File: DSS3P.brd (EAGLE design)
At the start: 399.7 x 251.8 mm, 299 parts, among them J1 J7MM

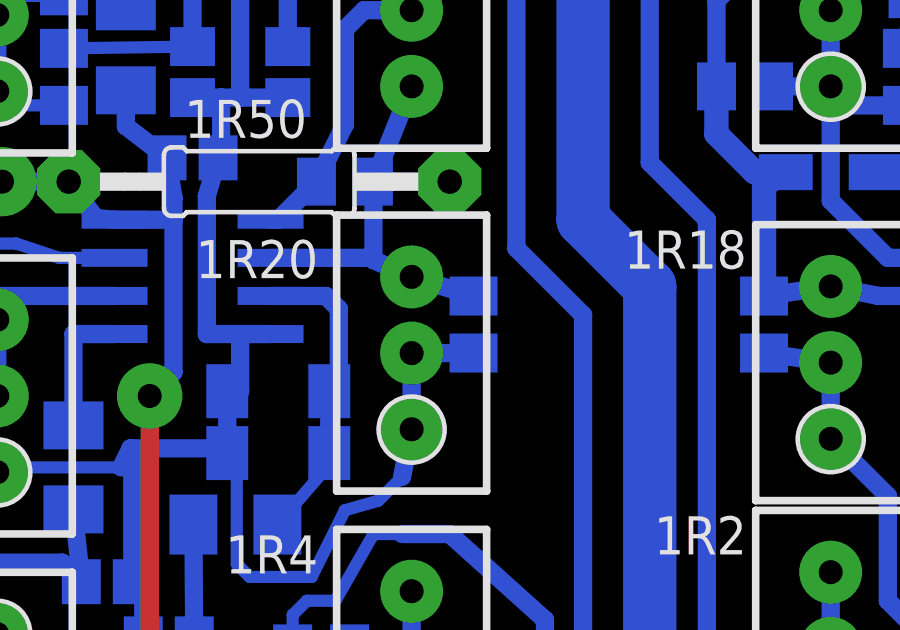
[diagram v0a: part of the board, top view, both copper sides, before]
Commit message: lab bot
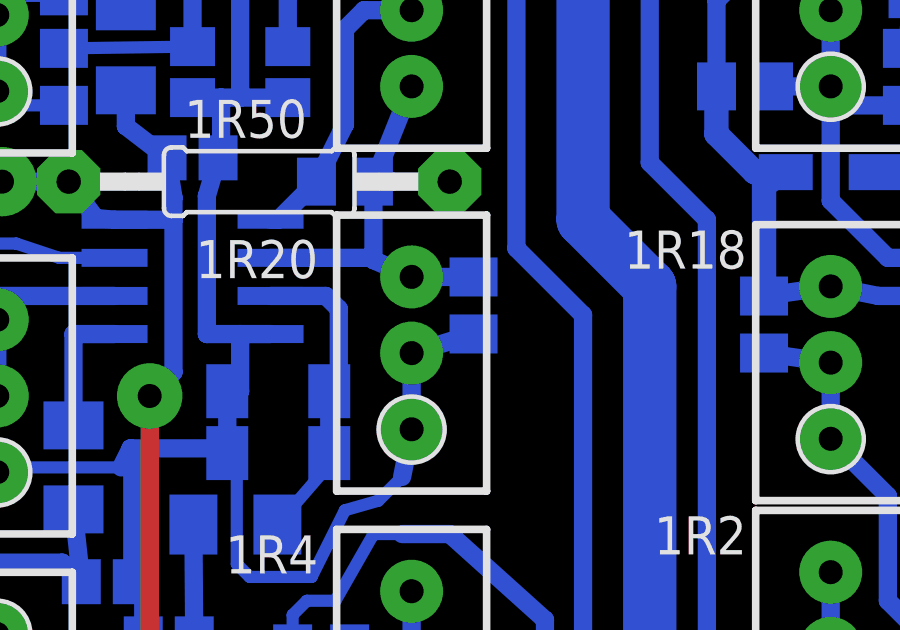
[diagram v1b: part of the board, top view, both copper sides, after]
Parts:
- moved 1R16 0.63 mm to (123.0, 83.5)
